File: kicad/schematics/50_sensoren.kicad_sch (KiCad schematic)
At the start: 0 parts

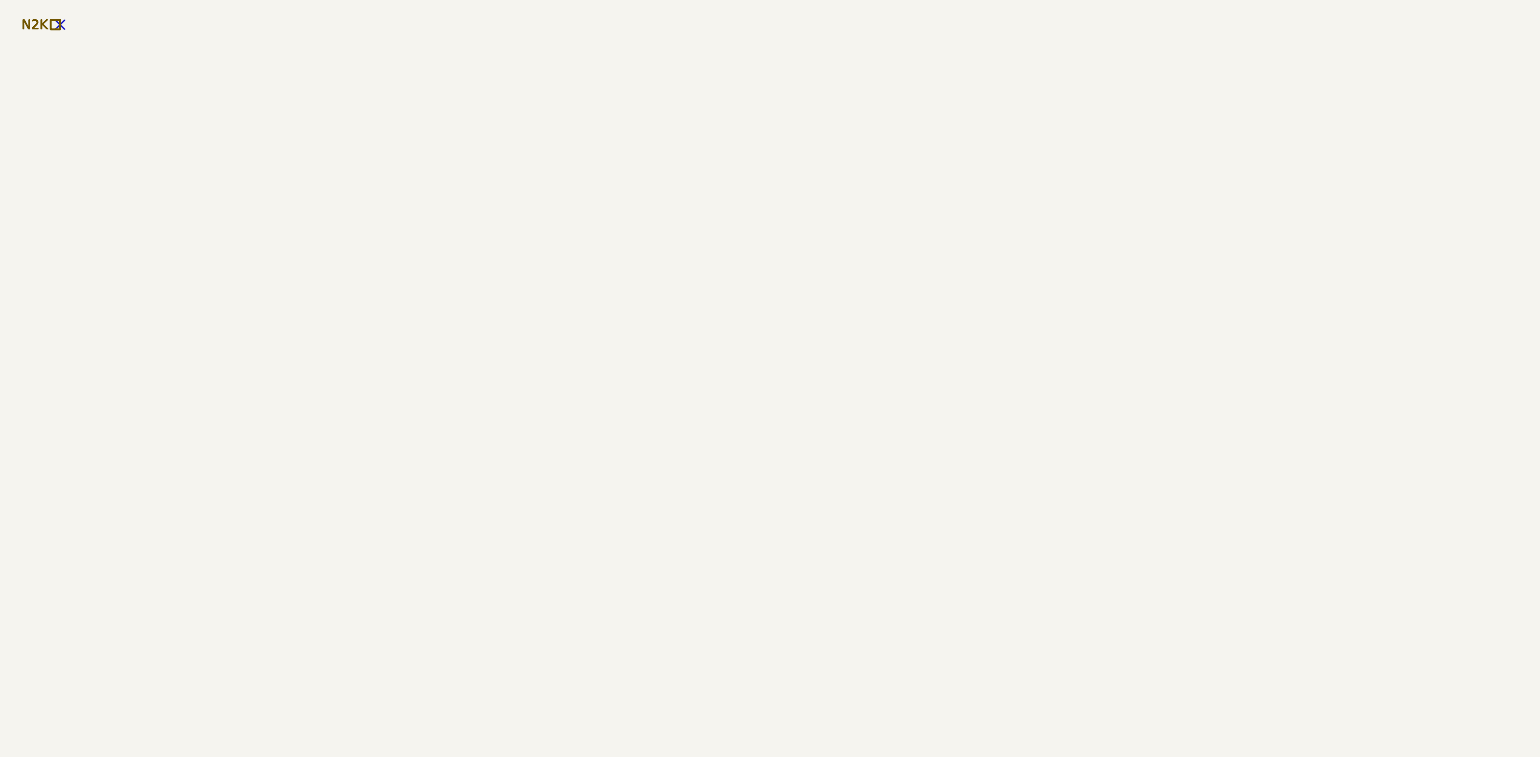
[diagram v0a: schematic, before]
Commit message: Schema's
00 toplevel stabiel
10 wisselstroom met subbladen stabiel
15 energieconversie stabiel
31 motor kern stabiel
32 motor sensoren stabiel
50 sensoren stabiel
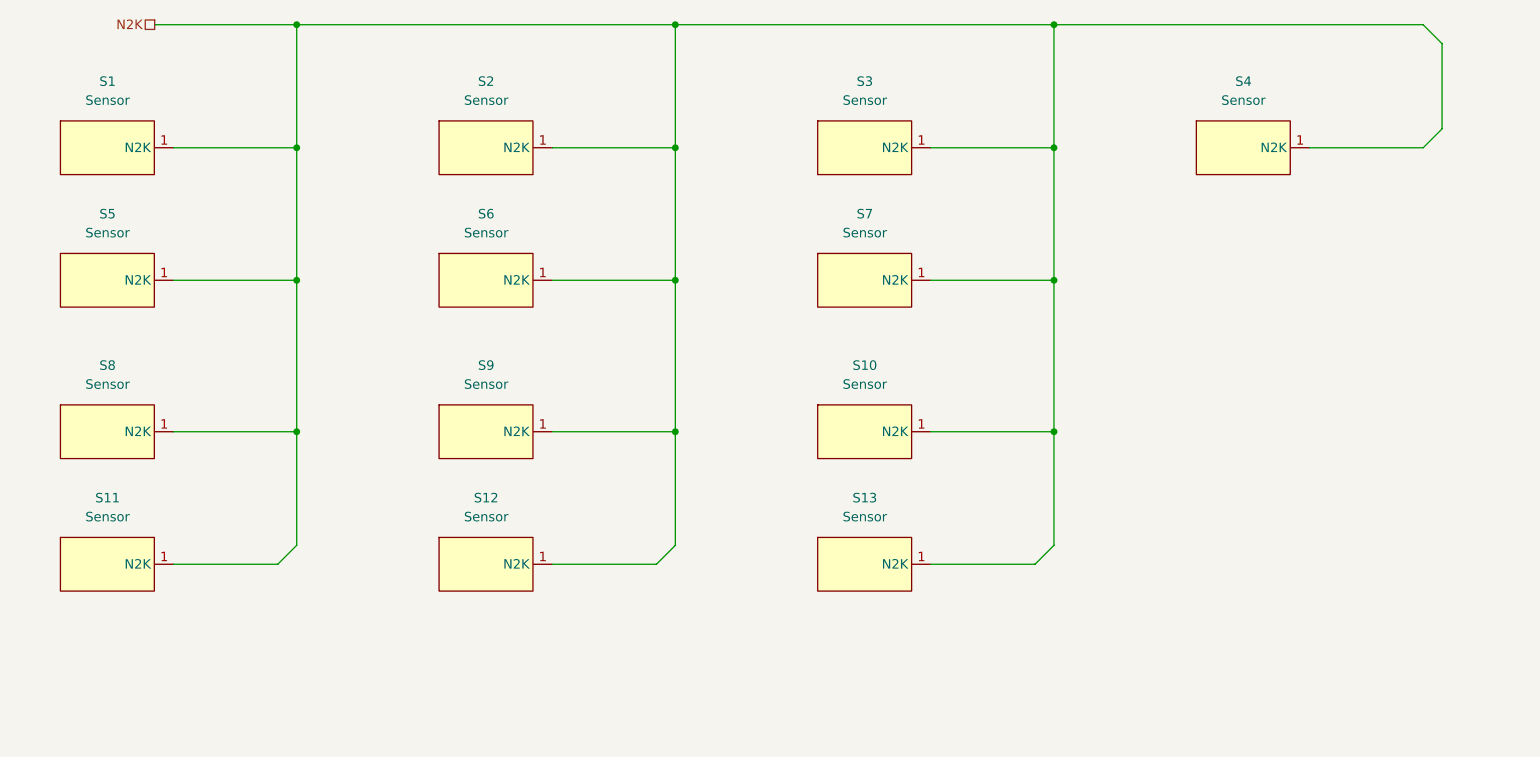
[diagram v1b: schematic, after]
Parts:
- added S1, S10, S11, S12, S13, S2, S3, S4, S5, S6, S7, S8, S9: Sensor, symbol falkor-electrical:sensor_n2k
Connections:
- net N2K: now also S1.1 (N2K), S10.1 (N2K), S11.1 (N2K), S12.1 (N2K), S13.1 (N2K), S2.1 (N2K), S3.1 (N2K), S4.1 (N2K), S5.1 (N2K), S6.1 (N2K), S7.1 (N2K), S8.1 (N2K), S9.1 (N2K)
- no-connect marks 1 -> 0

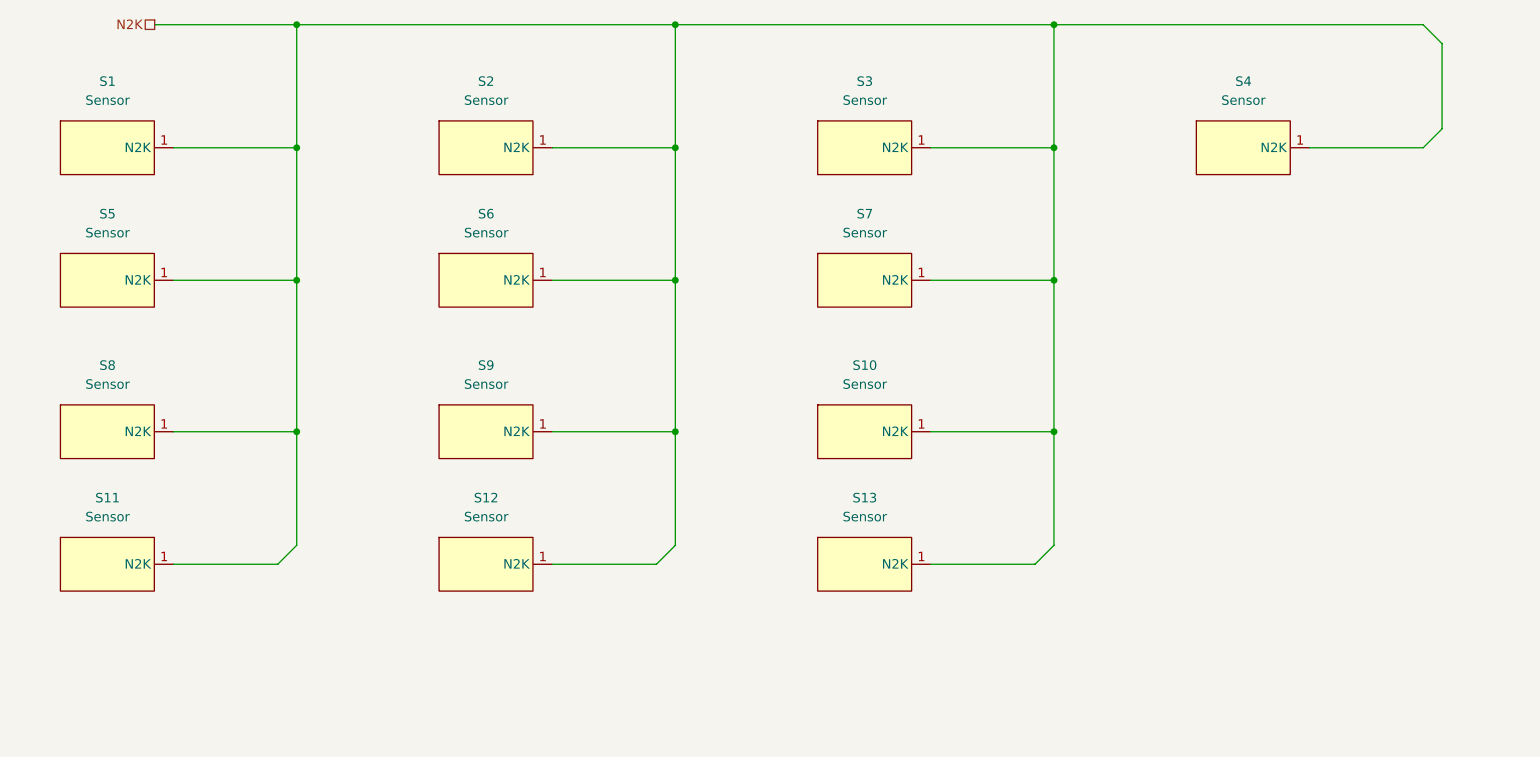
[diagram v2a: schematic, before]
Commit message: eerste opzet 21_laden_opslag_distributie
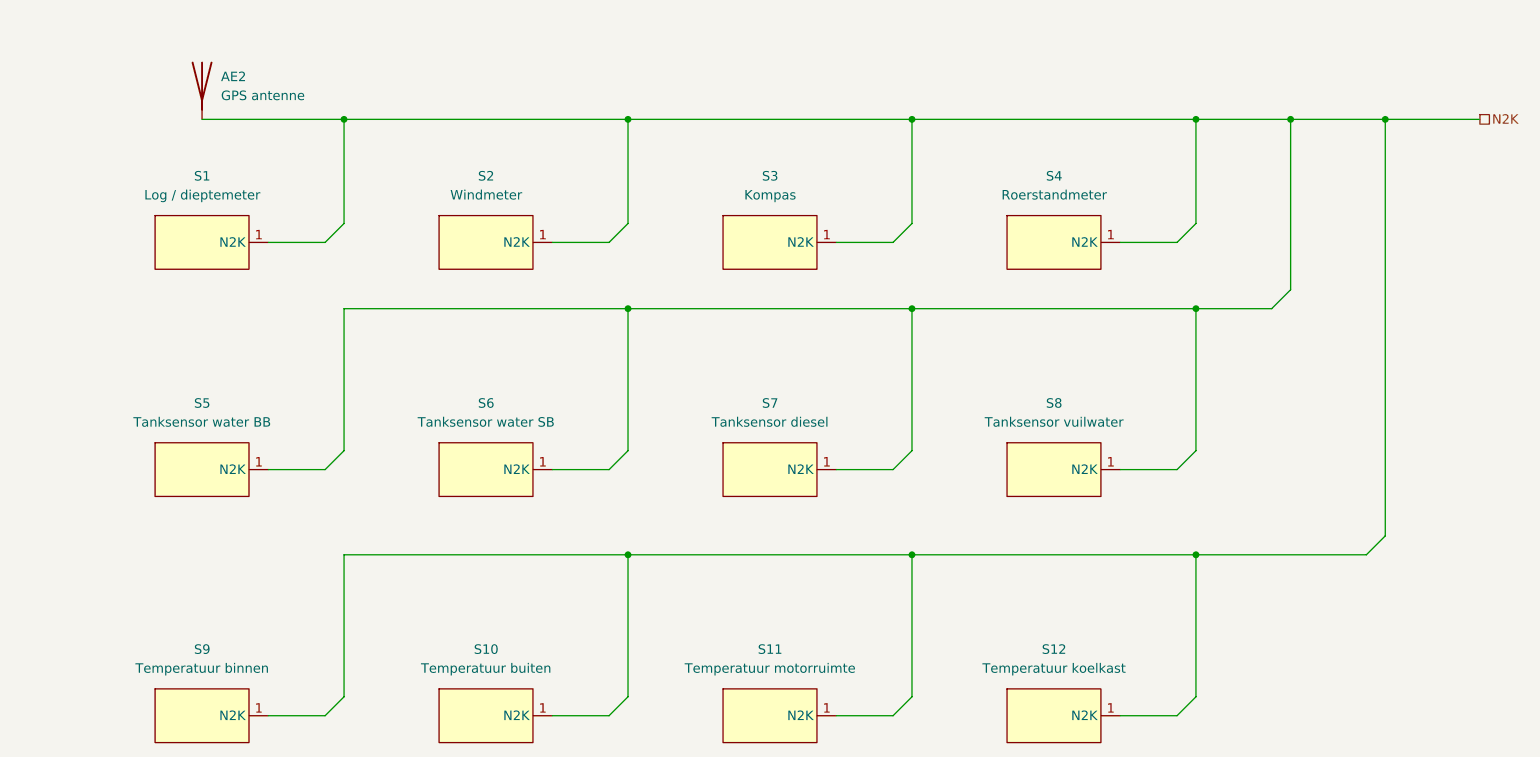
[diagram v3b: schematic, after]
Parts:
- removed S1, S13, S3, S7: Sensor, symbol falkor-electrical:sensor_n2k
- added AE2: GPS antenne, symbol Device:Antenna
- added S11: Temperatuur motorruimte, symbol falkor-electrical:sensor_n2k
- added S12: Temperatuur koelkast, symbol falkor-electrical:sensor_n2k
- added S9: Temperatuur binnen, symbol falkor-electrical:sensor_n2k
- S1: renamed from S5; value Sensor -> Log / dieptemeter
- S10: value Sensor -> Temperatuur buiten
- S2: renamed from S8; value Sensor -> Windmeter
- S3: renamed from S11; value Sensor -> Kompas
- S4: renamed from S2; value Sensor -> Roerstandmeter
- S5: renamed from S6; value Sensor -> Tanksensor water BB
- S6: renamed from S9; value Sensor -> Tanksensor water SB
- S7: renamed from S12; value Sensor -> Tanksensor diesel
- S8: renamed from S4; value Sensor -> Tanksensor vuilwater
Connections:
- net N2K: now also AE2.1 (A), S11.1 (N2K), S12.1 (N2K), S9.1 (N2K)
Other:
- moved on the sheet: S1, S2, S3, S4, S5, S6, S7, S8
